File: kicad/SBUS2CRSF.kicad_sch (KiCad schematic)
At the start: 5 parts, among them U1 ESP32-C3-SuperMini

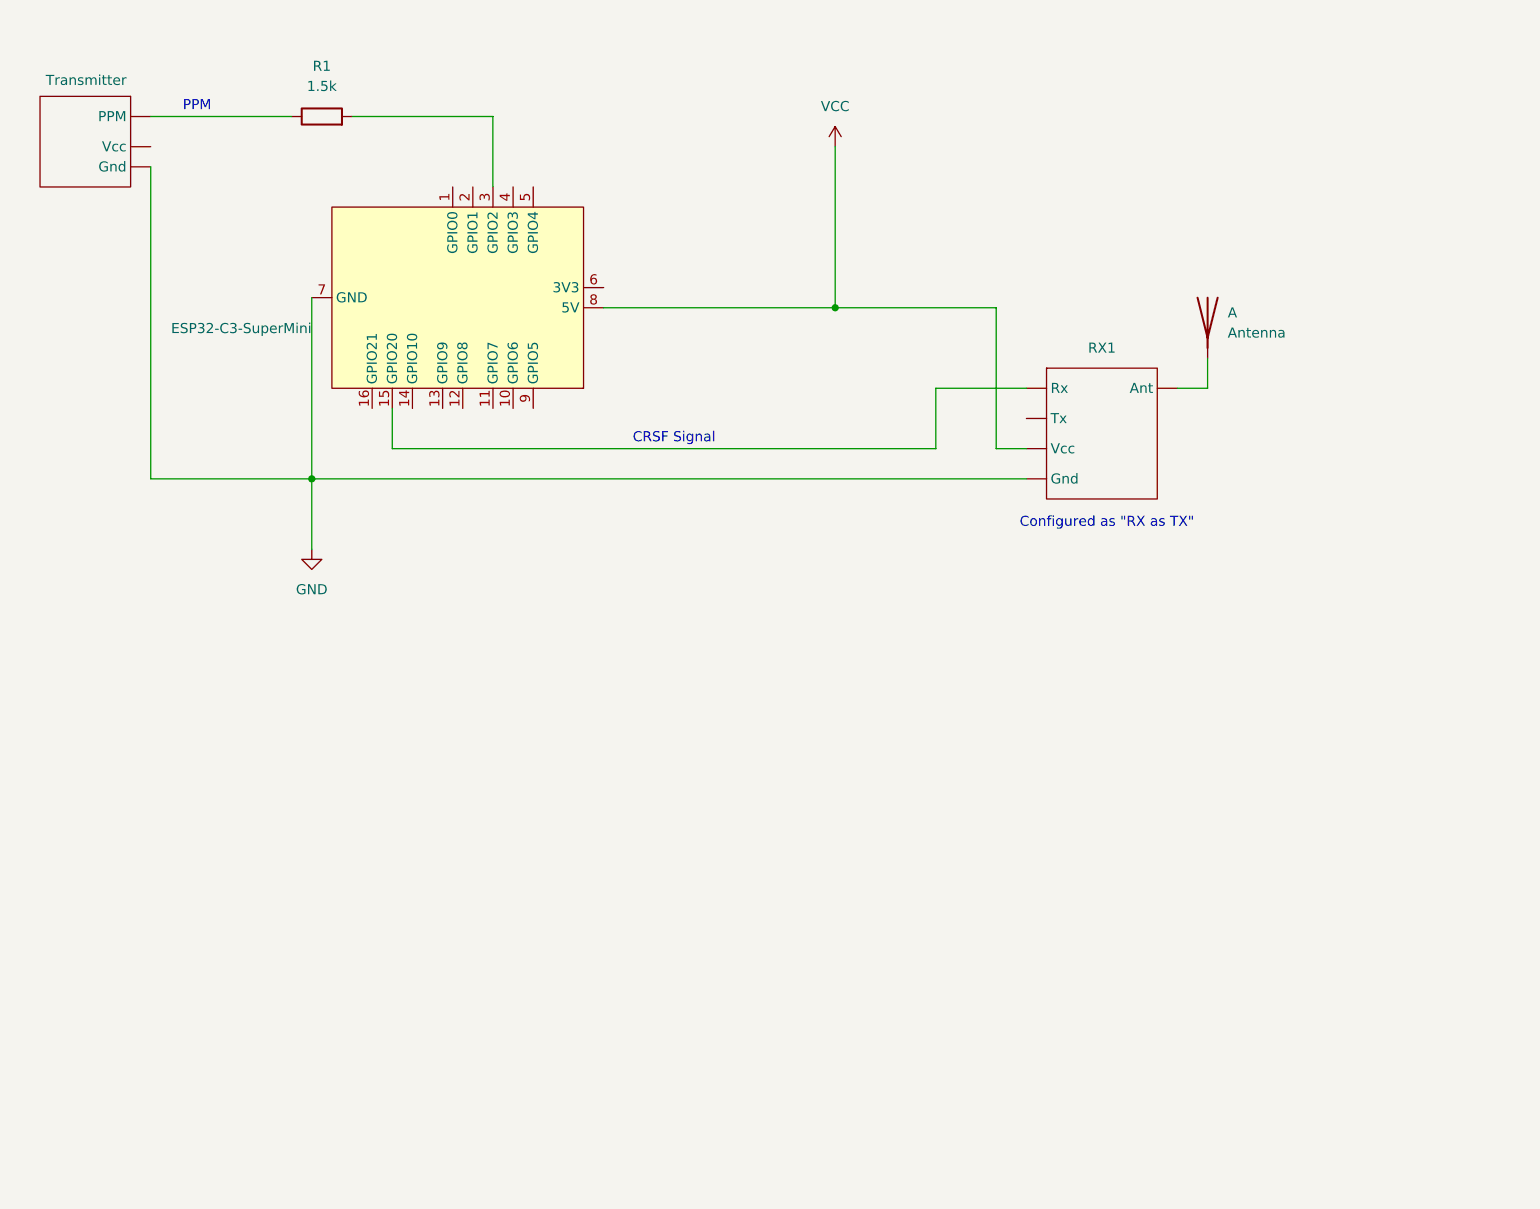
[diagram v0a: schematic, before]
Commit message: Updated KiCad files
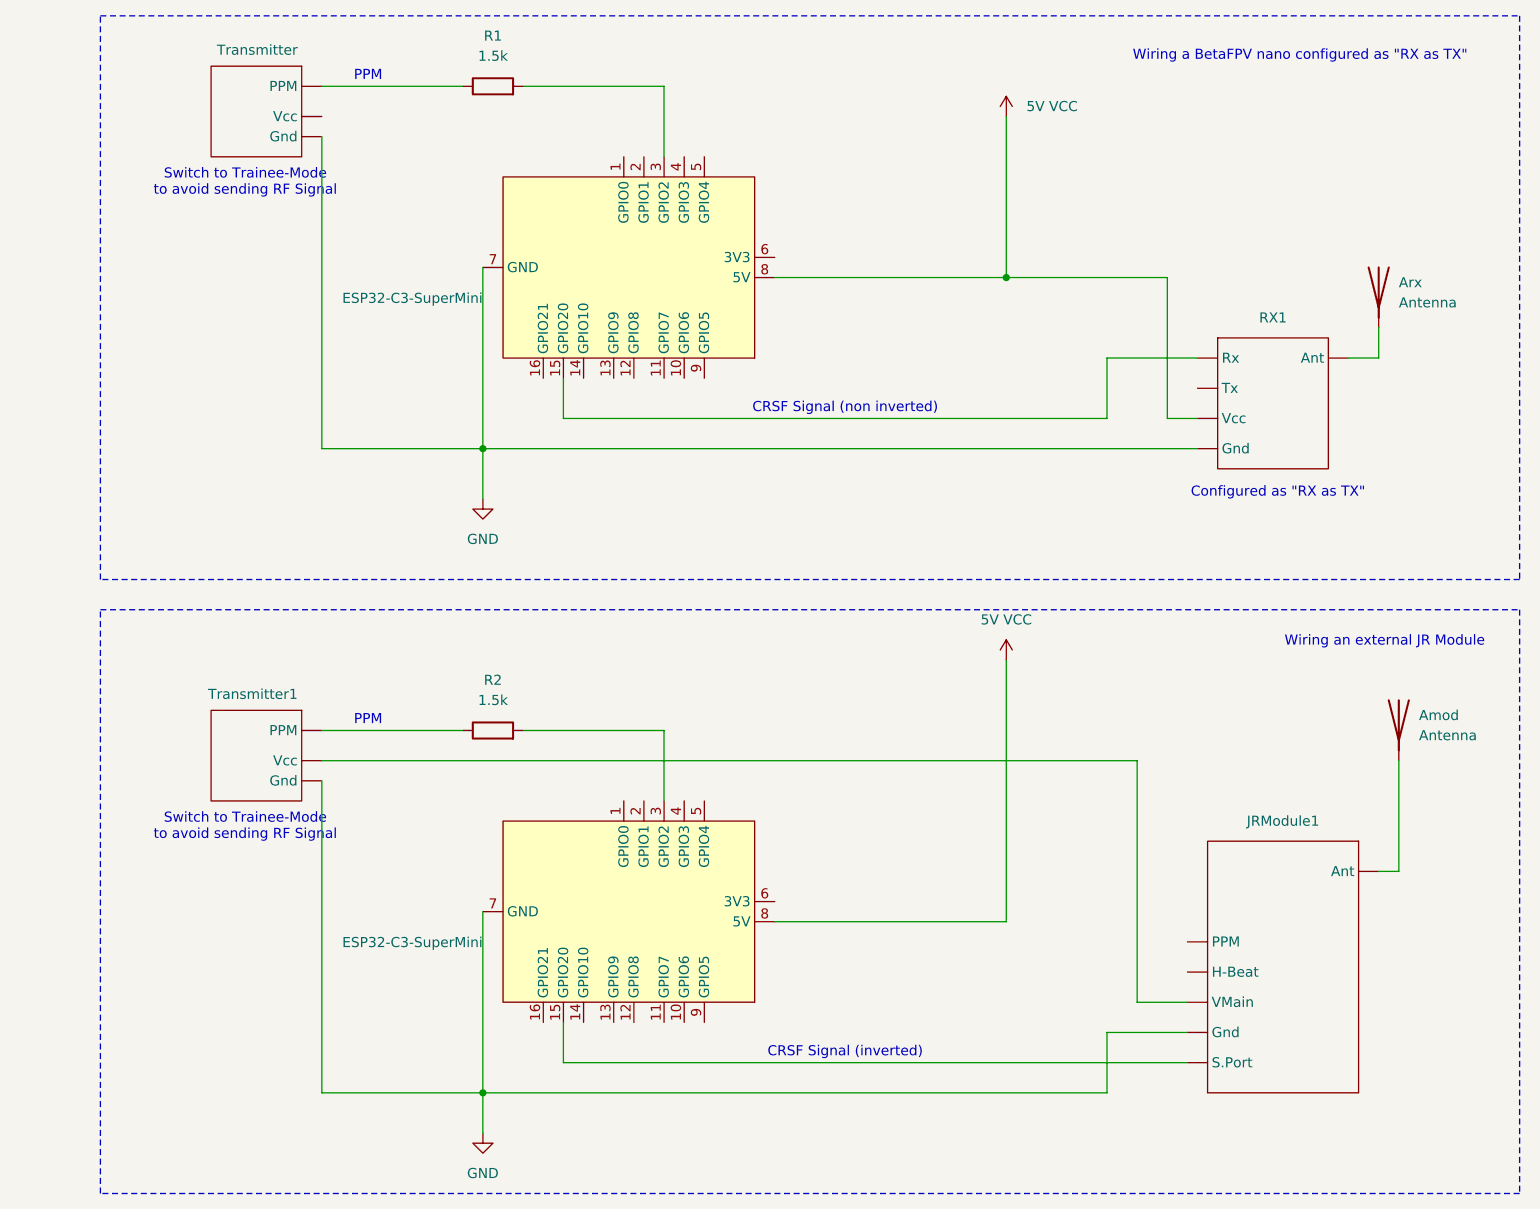
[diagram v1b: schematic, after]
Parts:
- added Amod: Antenna, symbol Device:Antenna
- added JRModule1: (no value), symbol icebreaker:JR
- added R2: 1.5k, symbol Device:R
- added Transmitter1: (no value), symbol Icebreaker:Transmitter
- added U2: ESP32-C3-SuperMini, ESP32-C3-SuperMini:ESP32-C3-SuperMini, symbol ESP32-C3-SuperMini:ESP32-C3-SuperMini
- renumbered A to Arx
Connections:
- net GND: now also JRModule1. (S.Port), Transmitter1. (Gnd), U2.7 (GND)
- net VCC renamed 5V VCC
- net 5V VCC: now also U2.8 (5V)
- new net: R2.1, Transmitter1. (Gnd)
- new net: R2.2, U2.3 (GPIO2)
- new net: JRModule1. (S.Port), U2.15 (GPIO20)
- new net: JRModule1. (S.Port), Transmitter1. (Gnd)
- new net: Amod.1 (A), JRModule1. (S.Port)
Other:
- note added: "CRSF Signal (inverted)"
- note added: "CRSF Signal (non inverted)"
- note added: "Switch to Trainee-Mode to avoid sending RF Signal"
- note added: "Wiring a BetaFPV nano configured as "RX as TX""
- note added: "Wiring an external JR Module"
- note removed: "CRSF Signal"
- moved on the sheet: Arx, R1, RX1, Transmitter
